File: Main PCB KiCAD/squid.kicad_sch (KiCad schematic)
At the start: 3 parts, among them U3 ESP32-S2-WROVER

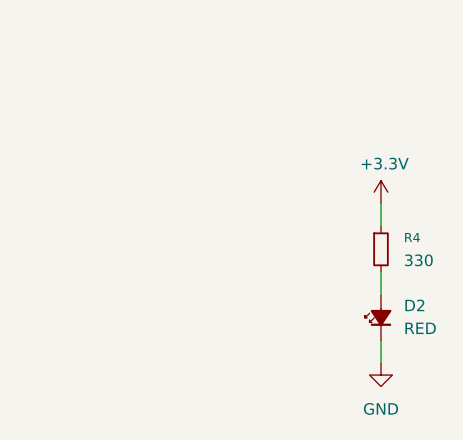
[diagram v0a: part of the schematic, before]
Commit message: this is likely to break all the things…
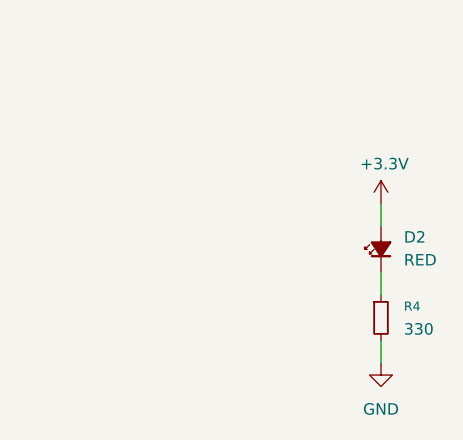
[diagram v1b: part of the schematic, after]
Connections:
- net +3.3V: now also D2.2 (A); no longer R4.1
- net GND: now also R4.2; no longer D2.1 (K)
- new net: D2.1 (K), R4.1
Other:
- moved on the sheet: D2, R4
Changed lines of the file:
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@@
 	(symbol
 		(lib_id "Device:R_Small")
-		(at 204.47 106.68 0)
+		(at 204.47 114.3 0)
 		(unit 1)
 		(exclude_from_sim no)
@@
 		(fields_autoplaced yes)
 		(property "Reference" "R4"
-			(at 207.01 105.4099 0)
+			(at 207.01 113.0299 0)
 			(effects
 				(font
@@
 		)
 		(property "Value" "330"
-			(at 207.01 107.9499 0)
+			(at 207.01 115.5699 0)
 			(effects
 				(font
@@
 		)
 		(property "Footprint" "Resistor_SMD:R_0805_2012Metric_Pad1.20x1.40mm_HandSolder"
-			(at 204.47 106.68 0)
+			(at 204.47 114.3 0)
 			(effects
 				(font
@@
 		)
 		(property "Datasheet" "~"
-			(at 204.47 106.68 0)
+			(at 204.47 114.3 0)
 			(effects
 				(font
@@
 		)
 		(property "Description" "Resistor, small symbol"
-			(at 204.47 106.68 0)
+			(at 204.47 114.3 0)
 			(effects
 				(font
@@
 	(symbol
 		(lib_id "Device:LED_Small_Filled")
-		(at 204.47 114.3 90)
+		(at 204.47 106.68 90)
 		(unit 1)
 		(exclude_from_sim no)
@@
 		(fields_autoplaced yes)
 		(property "Reference" "D2"
-			(at 207.01 112.9664 90)
+			(at 207.01 105.3464 90)
 			(effects
 				(font
@@
 		)
 		(property "Value" "RED"
-			(at 207.01 115.5064 90)
+			(at 207.01 107.8864 90)
 			(effects
 				(font
@@
 		)
 		(property "Footprint" "LED_SMD:LED_0805_2012Metric_Pad1.15x1.40mm_HandSolder"
-			(at 204.47 114.3 90)
+			(at 204.47 106.68 90)
 			(effects
 				(font
@@
 		)
 		(property "Datasheet" "~"
-			(at 204.47 114.3 90)
+			(at 204.47 106.68 90)
 			(effects
 				(font
@@
 		)
 		(property "Description" "Light emitting diode, small symbol, filled shape"
-			(at 204.47 114.3 0)
+			(at 204.47 106.68 0)
 			(effects
 				(font
@@
 		)
 		(property "Sim.Pins" "1=K 2=A"
-			(at 204.47 114.3 0)
+			(at 204.47 106.68 0)
 			(effects
 				(font

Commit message: clean
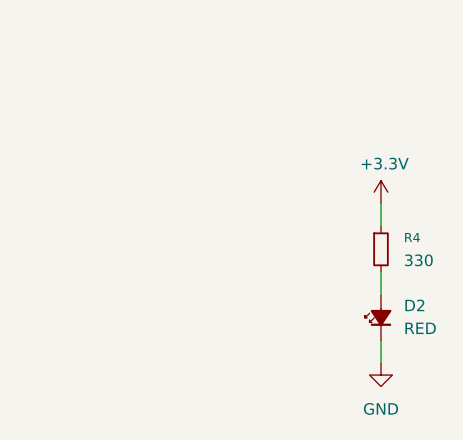
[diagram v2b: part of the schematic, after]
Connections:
- net +3.3V: now also R4.1; no longer D2.2 (A)
- net GND: now also D2.1 (K); no longer R4.2
- new net: D2.2 (A), R4.2
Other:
- moved on the sheet: D2, R4
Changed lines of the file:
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@@
 	(symbol
 		(lib_id "Device:R_Small")
-		(at 204.47 114.3 0)
+		(at 204.47 106.68 0)
 		(unit 1)
 		(exclude_from_sim no)
@@
 		(fields_autoplaced yes)
 		(property "Reference" "R4"
-			(at 207.01 113.0299 0)
+			(at 207.01 105.4099 0)
 			(effects
 				(font
@@
 		)
 		(property "Value" "330"
-			(at 207.01 115.5699 0)
+			(at 207.01 107.9499 0)
 			(effects
 				(font
@@
 		)
 		(property "Footprint" "Resistor_SMD:R_0805_2012Metric_Pad1.20x1.40mm_HandSolder"
-			(at 204.47 114.3 0)
+			(at 204.47 106.68 0)
 			(effects
 				(font
@@
 		)
 		(property "Datasheet" "~"
-			(at 204.47 114.3 0)
+			(at 204.47 106.68 0)
 			(effects
 				(font
@@
 		)
 		(property "Description" "Resistor, small symbol"
-			(at 204.47 114.3 0)
+			(at 204.47 106.68 0)
 			(effects
 				(font
@@
 	(symbol
 		(lib_id "Device:LED_Small_Filled")
-		(at 204.47 106.68 90)
+		(at 204.47 114.3 90)
 		(unit 1)
 		(exclude_from_sim no)
@@
 		(fields_autoplaced yes)
 		(property "Reference" "D2"
-			(at 207.01 105.3464 90)
+			(at 207.01 112.9664 90)
 			(effects
 				(font
@@
 		)
 		(property "Value" "RED"
-			(at 207.01 107.8864 90)
+			(at 207.01 115.5064 90)
 			(effects
 				(font
@@
 		)
 		(property "Footprint" "LED_SMD:LED_0805_2012Metric_Pad1.15x1.40mm_HandSolder"
-			(at 204.47 106.68 90)
+			(at 204.47 114.3 90)
 			(effects
 				(font
@@
 		)
 		(property "Datasheet" "~"
-			(at 204.47 106.68 90)
+			(at 204.47 114.3 90)
 			(effects
 				(font
@@
 		)
 		(property "Description" "Light emitting diode, small symbol, filled shape"
-			(at 204.47 106.68 0)
+			(at 204.47 114.3 0)
 			(effects
 				(font
@@
 		)
 		(property "Sim.Pins" "1=K 2=A"
-			(at 204.47 106.68 0)
+			(at 204.47 114.3 0)
 			(effects
 				(font
